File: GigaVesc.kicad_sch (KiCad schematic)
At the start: 26 parts, among them SW1 BOOT, SW2 RST, U1 STM32F405RGT7, U2 REF1933AIDDCT, Y1 Crystal

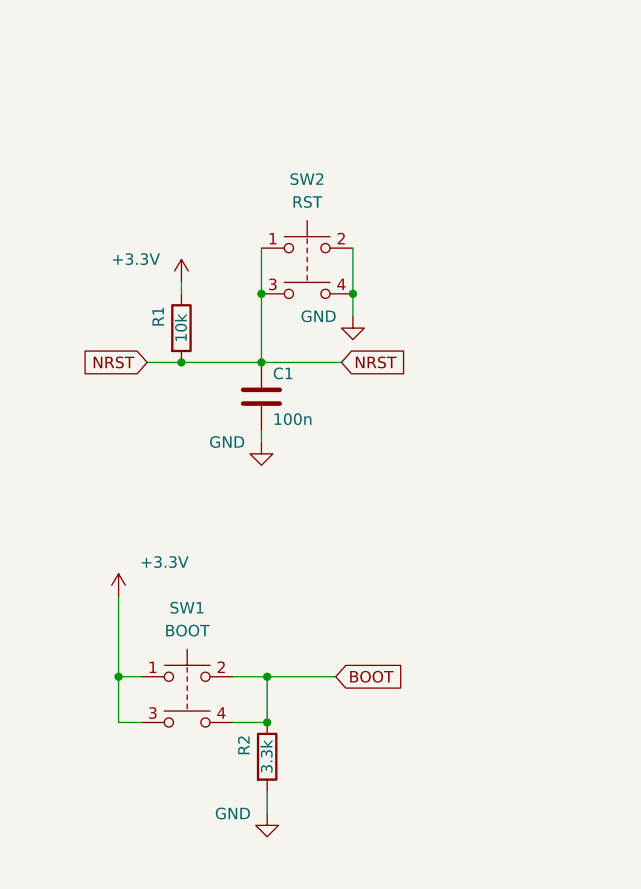
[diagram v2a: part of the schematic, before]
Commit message: jlcpcb
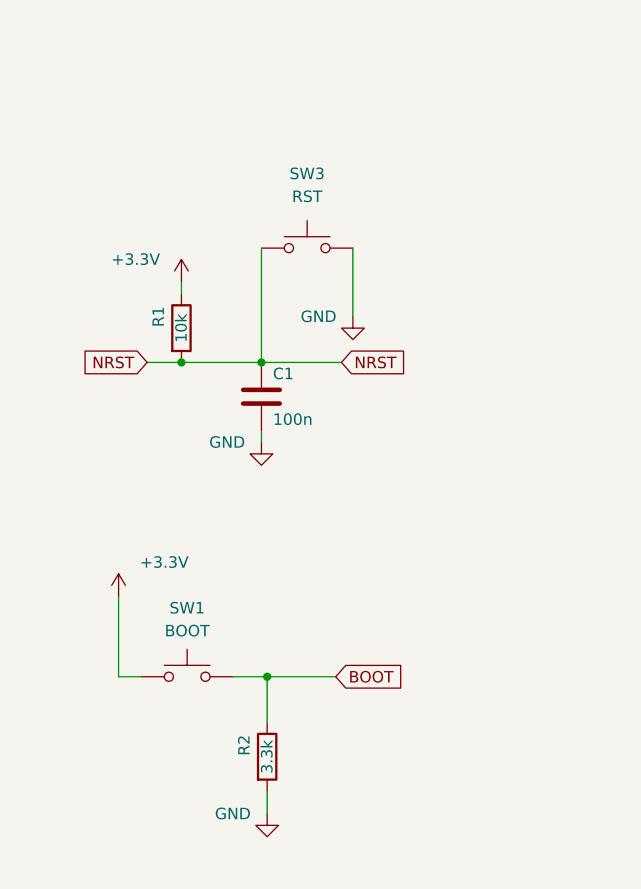
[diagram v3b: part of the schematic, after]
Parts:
- removed SW1: BOOT, Button_Switch_SMD:SW_SPST_CK_RS282G05A3, symbol Switch:SW_Push_Dual
- removed SW2: RST, Button_Switch_SMD:SW_SPST_CK_RS282G05A3, symbol Switch:SW_Push_Dual
- added SW1: BOOT, Button_Switch_SMD:SW_SPST_Omron_B3FS-100xP, symbol Switch:SW_Push
- added SW3: RST, Button_Switch_SMD:SW_SPST_Omron_B3FS-100xP, symbol Switch:SW_Push
- C1: MPN (none) -> C282732
- C10: MPN (none) -> C83170
- C14: MPN (none) -> C28323
- C2: MPN (none) -> C520056
- D1: MPN (none) -> C434435
- D2: MPN (none) -> C131244
- R1: MPN (none) -> C2930231
- R2: MPN (none) -> C114531
- U1: MPN (none) -> C1337199
- U2: MPN (none) -> C2877564
- Y1: MPN (none) -> C12674
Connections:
- net +3.3V: now also SW1.1
- net BOOT: now also SW1.2
- net GND: now also SW3.2
- net NRST: now also SW3.1
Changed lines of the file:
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@@
   (junction (at 143.51 78.74) (diameter 0) (color 0 0 0 0)
   )
-  (junction (at 48.895 137.16) (diameter 0) (color 0 0 0 0)
-  )
   (junction (at 113.03 99.06) (diameter 0) (color 0 0 0 0)
   )
-  (junction (at 48.26 89.535) (diameter 0) (color 0 0 0 0)
-  )
   (junction (at 226.06 133.35) (diameter 0) (color 0 0 0 0)
   )
@@
   (junction (at 39.37 97.155) (diameter 0) (color 0 0 0 0)
   )
-  (junction (at 32.385 132.08) (diameter 0) (color 0 0 0 0)
-  )
   (junction (at 140.97 64.77) (diameter 0) (color 0 0 0 0)
   )
   (junction (at 146.05 175.26) (diameter 0) (color 0 0 0 0)
-  )
-  (junction (at 58.42 89.535) (diameter 0) (color 0 0 0 0)
   )
   (junction (at 113.03 91.44) (diameter 0) (color 0 0 0 0)
@@
     (stroke (width 0) (type default))
   )
-  (wire (pts (xy 32.385 137.16) (xy 34.925 137.16))
-    (stroke (width 0) (type default))
-  )
   (wire (pts (xy 140.97 78.74) (xy 143.51 78.74))
     (stroke (width 0) (type default))
@@
     (stroke (width 0) (type default))
   )
-  (wire (pts (xy 45.085 137.16) (xy 48.895 137.16))
-    (stroke (width 0) (type default))
-  )
   (wire (pts (xy 113.03 52.07) (xy 113.03 57.15))
     (stroke (width 0) (type default))
@@
     (stroke (width 0) (type default))
   )
-  (wire (pts (xy 48.26 84.455) (xy 48.26 89.535))
+  (wire (pts (xy 48.26 84.455) (xy 48.26 97.155))
     (stroke (width 0) (type default))
   )
@@
     (stroke (width 0) (type default))
   )
-  (wire (pts (xy 32.385 132.08) (xy 32.385 137.16))
-    (stroke (width 0) (type default))
-  )
   (wire (pts (xy 163.83 157.48) (xy 167.64 157.48))
     (stroke (width 0) (type default))
@@
     (stroke (width 0) (type default))
   )
-  (wire (pts (xy 48.26 89.535) (xy 48.26 97.155))
-    (stroke (width 0) (type default))
-  )
   (wire (pts (xy 106.68 91.44) (xy 113.03 91.44))
     (stroke (width 0) (type default))
@@
     (stroke (width 0) (type default))
   )
-  (wire (pts (xy 58.42 84.455) (xy 58.42 89.535))
+  (wire (pts (xy 58.42 84.455) (xy 58.42 92.075))
     (stroke (width 0) (type default))
   )
@@
     (stroke (width 0) (type default))
   )
-  (wire (pts (xy 58.42 89.535) (xy 58.42 92.075))
-    (stroke (width 0) (type default))
-  )
   (wire (pts (xy 109.22 167.64) (xy 115.57 167.64))
     (stroke (width 0) (type default))
@@
         (path "/768a484b-8a27-40cf-8cad-0f63935b1af0"
           (reference "C15") (unit 1)
+        )
+      )
+    )
+  )
+  (symbol (lib_id "Switch:SW_Push") (at 40.005 132.08 0) (unit 1)
+    (in_bom yes) (on_board yes) (dnp no) (fields_autoplaced)
+    (property "Reference" "SW1" (at 40.005 124.46 0)
+      (effects (font (size 1.27 1.27)))
+    )
+    (property "Value" "BOOT" (at 40.005 127 0)
+      (effects (font (size 1.27 1.27)))
+    )
+    (property "Footprint" "Button_Switch_SMD:SW_SPST_Omron_B3FS-100xP" (at 40.005 127 0)
+      (effects (font (size 1.27 1.27)) hide)
+    )
+    (property "Datasheet" "~" (at 40.005 127 0)
+      (effects (font (size 1.27 1.27)) hide)
+    )
+    (property "MPN" "C271750" (at 40.005 132.08 0)
+      (effects (font (size 1.27 1.27)) hide)
+    )
+    (pin "1")
+    (pin "2")
+    (instances
+      (project "GigaVesc"
+        (path "/768a484b-8a27-40cf-8cad-0f63935b1af0"
+          (reference "SW1") (unit 1)
+        )
+      )
+    )
+  )
+  (symbol (lib_id "Switch:SW_Push") (at 53.34 84.455 0) (unit 1)
+    (in_bom yes) (on_board yes) (dnp no) (fields_autoplaced)
+    (property "Reference" "SW3" (at 53.34 76.2 0)
+      (effects (font (size 1.27 1.27)))
+    )
+    (property "Value" "RST" (at 53.34 78.74 0)
+      (effects (font (size 1.27 1.27)))
+    )
+    (property "Footprint" "Button_Switch_SMD:SW_SPST_Omron_B3FS-100xP" (at 53.34 79.375 0)
+      (effects (font (size 1.27 1.27)) hide)
+    )
+    (property "Datasheet" "~" (at 53.34 79.375 0)
+      (effects (font (size 1.27 1.27)) hide)
+    )
+    (property "MPN" "C271750" (at 53.34 84.455 0)
+      (effects (font (size 1.27 1.27)) hide)
+    )
+    (pin "1")
+    (pin "2")
+    (instances
+      (project "GigaVesc"
+        (path "/768a484b-8a27-40cf-8cad-0f63935b1af0"
+          (reference "SW3") (unit 1)
         )
       )
@@
       (effects (font (size 1.27 1.27)) hide)
     )
+    (property "MPN" "C28323" (at 226.06 139.7 0)
+      (effects (font (size 1.27 1.27)) hide)
+    )
     (pin "1")
     (pin "2")
@@
       (effects (font (size 1.27 1.27)) hide)
     )
+    (property "MPN" "C520056" (at 102.87 91.44 90)
+      (effects (font (size 1.27 1.27)) hide)
+    )
     (pin "1")
     (pin "2")
@@
       (effects (font (size 1.27 1.27)) hide)
     )
+    (property "MPN" "C2930231" (at 39.37 93.345 90)
+      (effects (font (size 1.27 1.27)) hide)
+    )
     (pin "1")
     (pin "2")
@@
       (effects (font (size 1.27 1.27)) hide)
     )
+    (property "MPN" "C83170" (at 152.4 60.96 0)
+      (effects (font (size 1.27 1.27)) hide)
+    )
     (pin "1")
     (pin "2")
@@
     )
     (property "Datasheet" "~" (at 48.26 100.965 0)
+      (effects (font (size 1.27 1.27)) hide)
+    )
+    (property "MPN" "C282732" (at 48.26 100.965 0)
       (effects (font (size 1.27 1.27)) hide)
     )
@@
       (effects (font (size 1.27 1.27)) hide)
     )
+    (property "MPN" "C434435" (at 41.91 173.99 90)
+      (effects (font (size 1.27 1.27)) hide)
+    )
     (pin "1")
     (pin "2")
@@
       (effects (font (size 1.27 1.27)) hide)
     )
+    (property "MPN" "C131244" (at 41.91 182.88 90)
+      (effects (font (size 1.27 1.27)) hide)
+    )
     (pin "1")
     (pin "2")
@@
     )
     (property "Datasheet" "" (at 246.38 135.89 0)
+      (effects (font (size 1.27 1.27)) hide)
+    )
+    (property "MPN" "C2877564" (at 246.38 135.89 0)
       (effects (font (size 1.27 1.27)) hide)
     )
@@
       (effects (font (size 1.27 1.27)) hide)
     )
+    (property "MPN" "C114531" (at 48.895 140.97 90)
+      (effects (font (size 1.27 1.27)) hide)
+    )
     (pin "1")
     (pin "2")
@@
         (path "/768a484b-8a27-40cf-8cad-0f63935b1af0"
           (reference "R2") (unit 1)
-        )
-      )
-    )
-  )
-  (symbol (lib_id "Switch:SW_Push_Dual") (at 53.34 84.455 0) (unit 1)
-    (in_bom yes) (on_board yes) (dnp no) (fields_autoplaced)
-    (property "Reference" "SW2" (at 53.34 76.835 0)
-      (effects (font (size 1.27 1.27)))
-    )
-    (property "Value" "RST" (at 53.34 79.375 0)
-      (effects (font (size 1.27 1.27)))
-    )
-    (property "Footprint" "Button_Switch_SMD:SW_SPST_CK_RS282G05A3" (at 53.34 79.375 0)
-      (effects (font (size 1.27 1.27)) hide)
-    )
-    (property "Datasheet" "~" (at 53.34 79.375 0)
-      (effects (font (size 1.27 1.27)) hide)
-    )
-    (pin "1")
-    (pin "2")
-    (pin "3")
-    (pin "4")
-    (instances
-      (project "GigaVesc"
-        (path "/768a484b-8a27-40cf-8cad-0f63935b1af0"
-          (reference "SW2") (unit 1)
         )
       )
@@
       (effects (font (size 1.27 1.27)) hide)
     )
+    (property "MPN" "C12674" (at 113.03 95.25 90)
+      (effects (font (size 1.27 1.27)) hide)
+    )
     (pin "1")
     (pin "2")
@@
     )
     (property "Datasheet" "https://www.st.com/resource/en/datasheet/stm32f405rg.pdf" (at 146.05 127 0)
+      (effects (font (size 1.27 1.27)) hide)
+    )
+    (property "MPN" "C1337199" (at 146.05 127 0)
       (effects (font (size 1.27 1.27)) hide)
     )
@@
         )
       )
-    )
-  )
-  (symbol (lib_id "Switch:SW_Push_Dual") (at 40.005 132.08 0) (unit 1)
-    (in_bom yes) (on_board yes) (dnp no) (fields_autoplaced)
-    (property "Reference" "SW1" (at 40.005 124.46 0)
-      (effects (font (size 1.27 1.27)))
-    )
-    (property "Value" "BOOT" (at 40.005 127 0)
-      (effects (font (size 1.27 1.27)))
-    )
-    (property "Footprint" "Button_Switch_SMD:SW_SPST_CK_RS282G05A3" (at 40.005 127 0)
-      (effects (font (size 1.27 1.27)) hide)
-    )
-    (property "Datasheet" "~" (at 40.005 127 0)
-      (effects (font (size 1.27 1.27)) hide)
-    )
-    (pin "1")
-    (pin "2")
-    (pin "3")
-    (pin "4")
-    (instances
-      (project "GigaVesc"
-        (path "/768a484b-8a27-40cf-8cad-0f63935b1af0"
-          (reference "SW1") (unit 1)
-        )
-      )

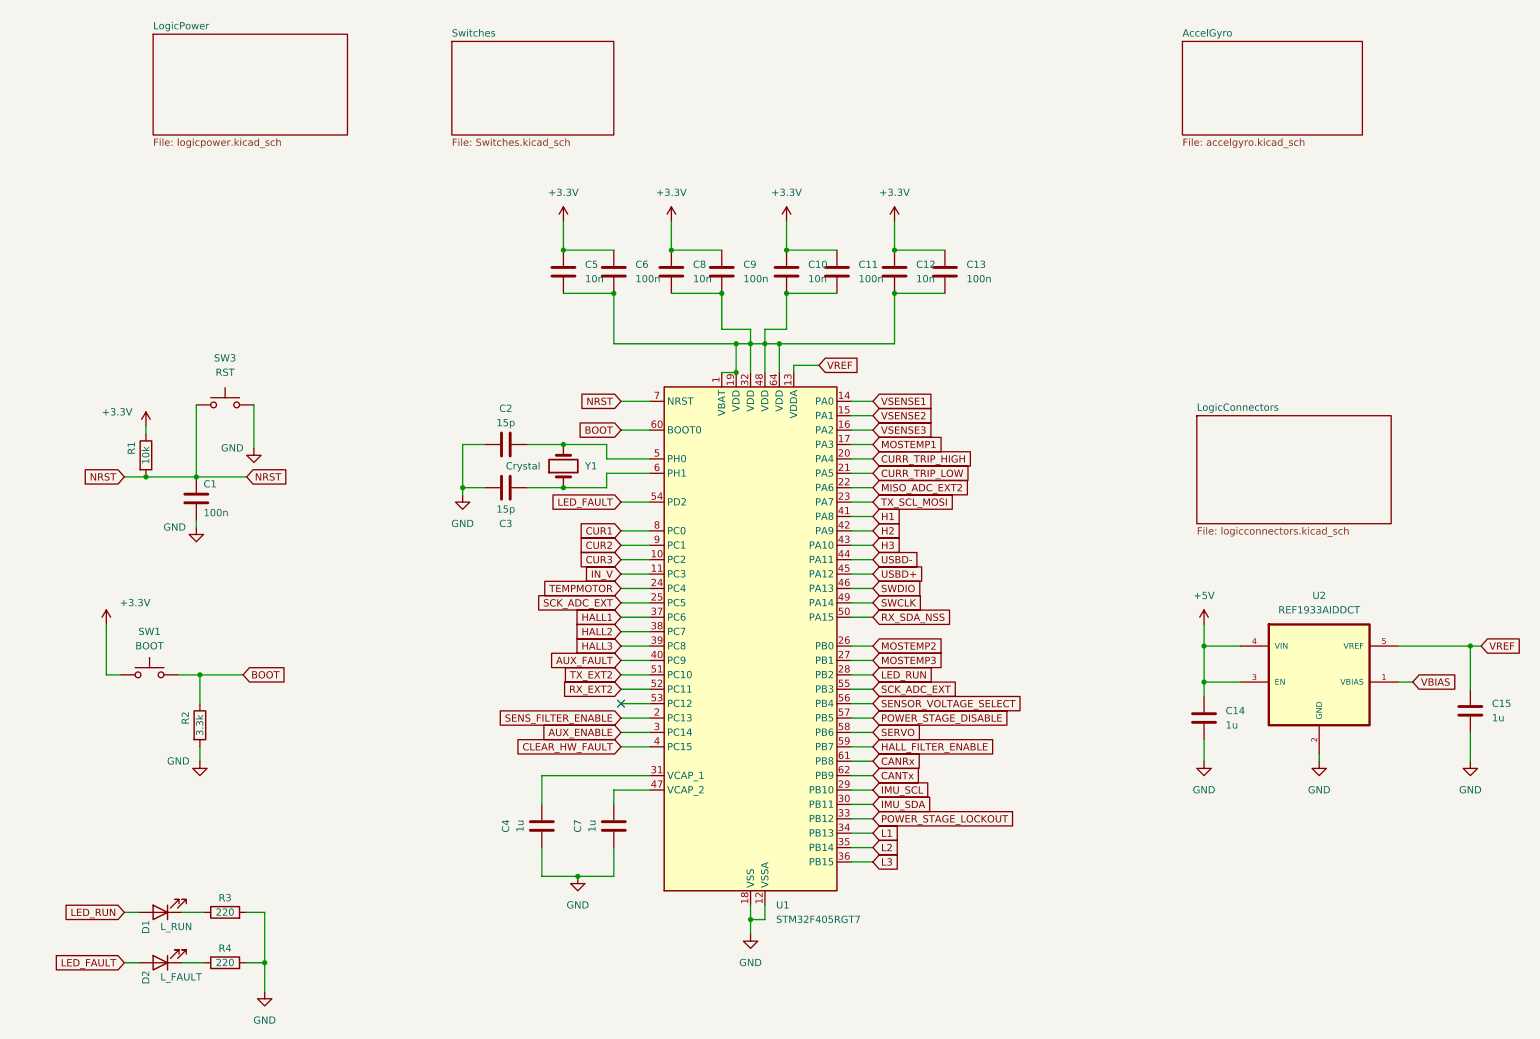
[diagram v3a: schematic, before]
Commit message: routinglogic
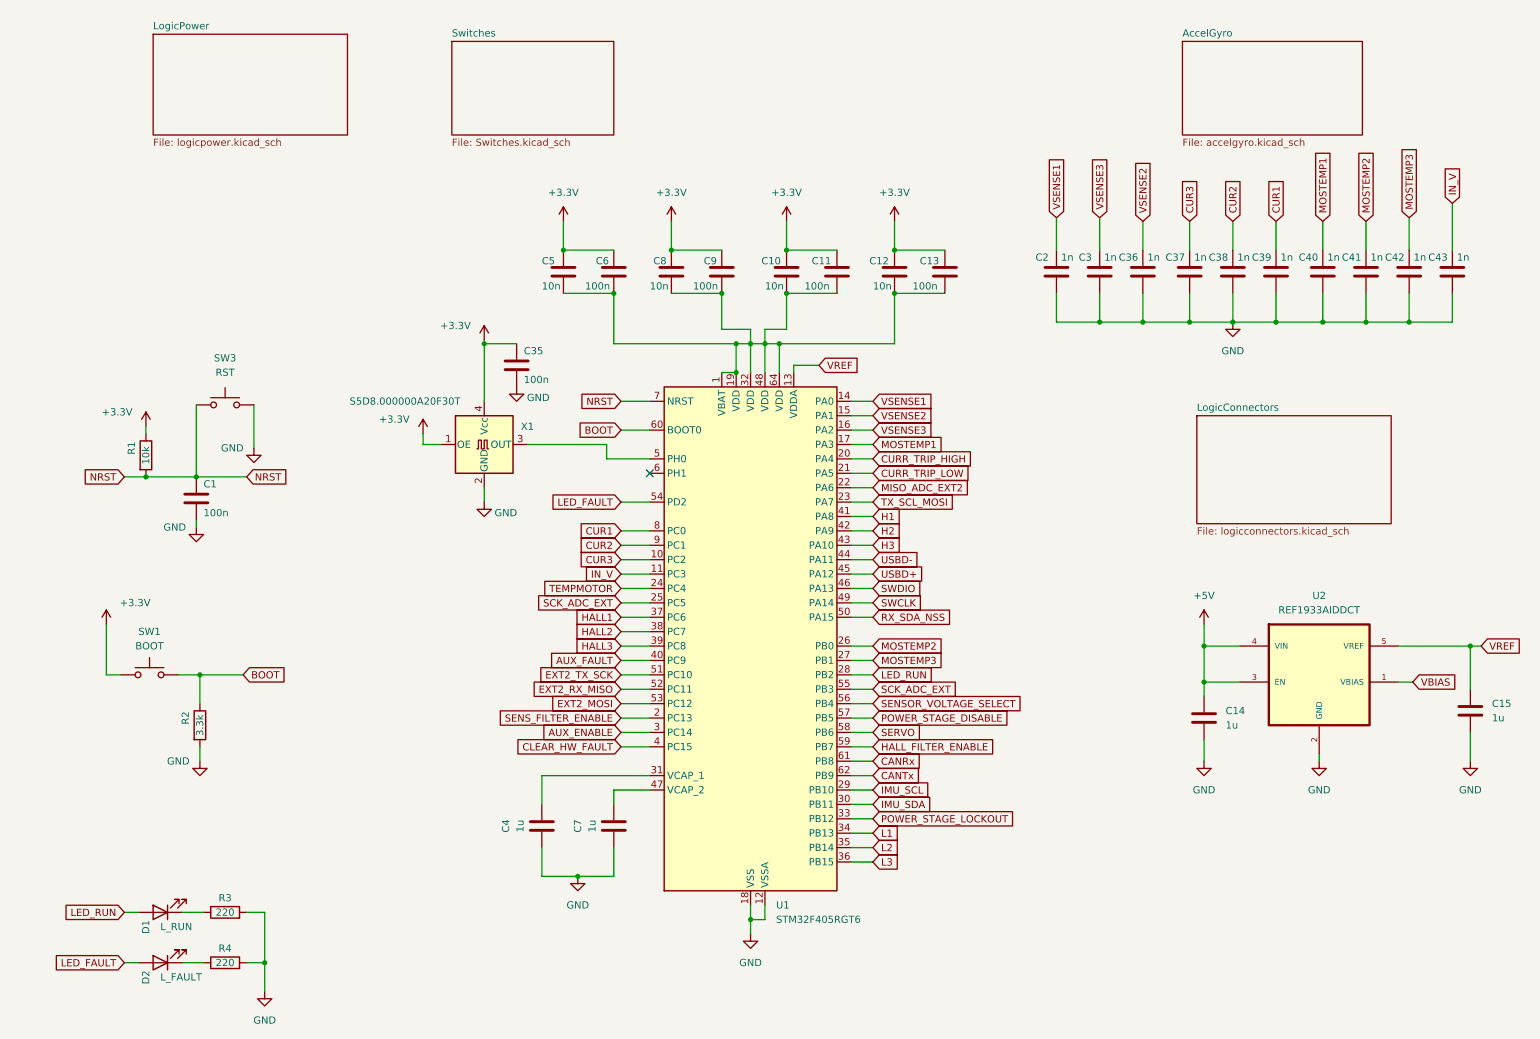
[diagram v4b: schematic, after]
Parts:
- removed Y1: Crystal, Crystal:Crystal_SMD_HC49-SD, symbol Device:Crystal
- added C35: 100n, Capacitor_SMD:C_0805_2012Metric, symbol Device:C
- added C36, C37, C38, C39, C40, C41, C42, C43: 1n, Capacitor_SMD:C_0805_2012Metric, symbol Device:C
- added X1: S5D8.000000A20F30T, Crystal:Crystal_SMD_5032-4Pin_5.0x3.2mm, symbol Oscillator:SG-5032CCN
- C2: value 15p -> 1n; MPN C520056 -> C94121
- C3: value 15p -> 1n; MPN (none) -> C94121
- U1: value STM32F405RGT7 -> STM32F405RGT6; JLCRotOffset (none) -> -90; MPN C1337199 -> C15742
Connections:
- net +3.3V: now also C35.1, X1.1 (OE), X1.4 (Vcc)
- net CUR1: now also C39.1
- net CUR2: now also C38.1
- net CUR3: now also C37.1
- net GND: now also C3.2, C35.2, C36.2, C37.2, C38.2, C39.2, C40.2, C41.2, C42.2, C43.2, X1.2 (GND); no longer C3.1
- net IN_V: now also C43.1
- net MOSTEMP1: now also C40.1
- net MOSTEMP2: now also C41.1
- net MOSTEMP3: now also C42.1
- net VSENSE1: now also C2.1
- net VSENSE2: now also C36.1
- net VSENSE3: now also C3.1
- net at U1.5 (PH0): now also X1.3 (OUT); no longer C2.1
- net at U1.6 (PH1): no longer C3.2
- net EXT2_MOSI: now reaches U1.53 (PC12)
- net RX_EXT2 renamed EXT2_RX_MISO
- net TX_EXT2 renamed EXT2_TX_SCK
